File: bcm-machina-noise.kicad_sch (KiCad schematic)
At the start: 61 parts, among them J1 USB_A, J2 AVR-ISP-6, J3 AudioJack2_Ground, J4 AudioJack2_Ground, Q1 2N5457, Q2 2N5457, SW1 SW_Push, SW2 SW_Push, U1 4069, U2 MCP602, U3 ATtiny84V-10P

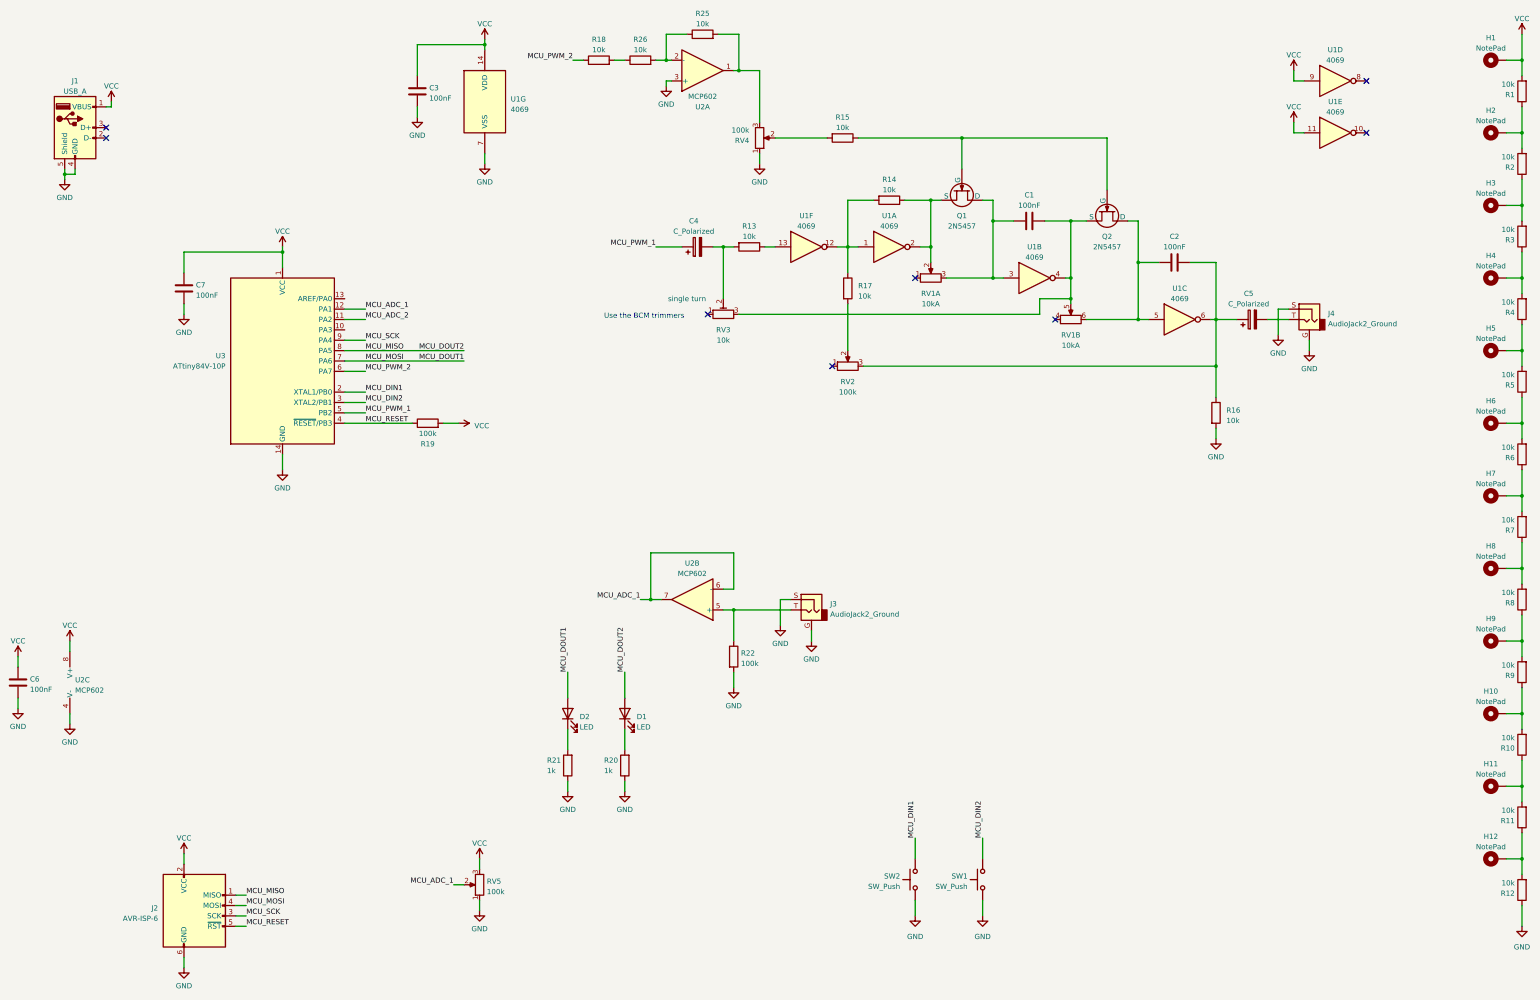
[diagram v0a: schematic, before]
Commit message: fixed errors
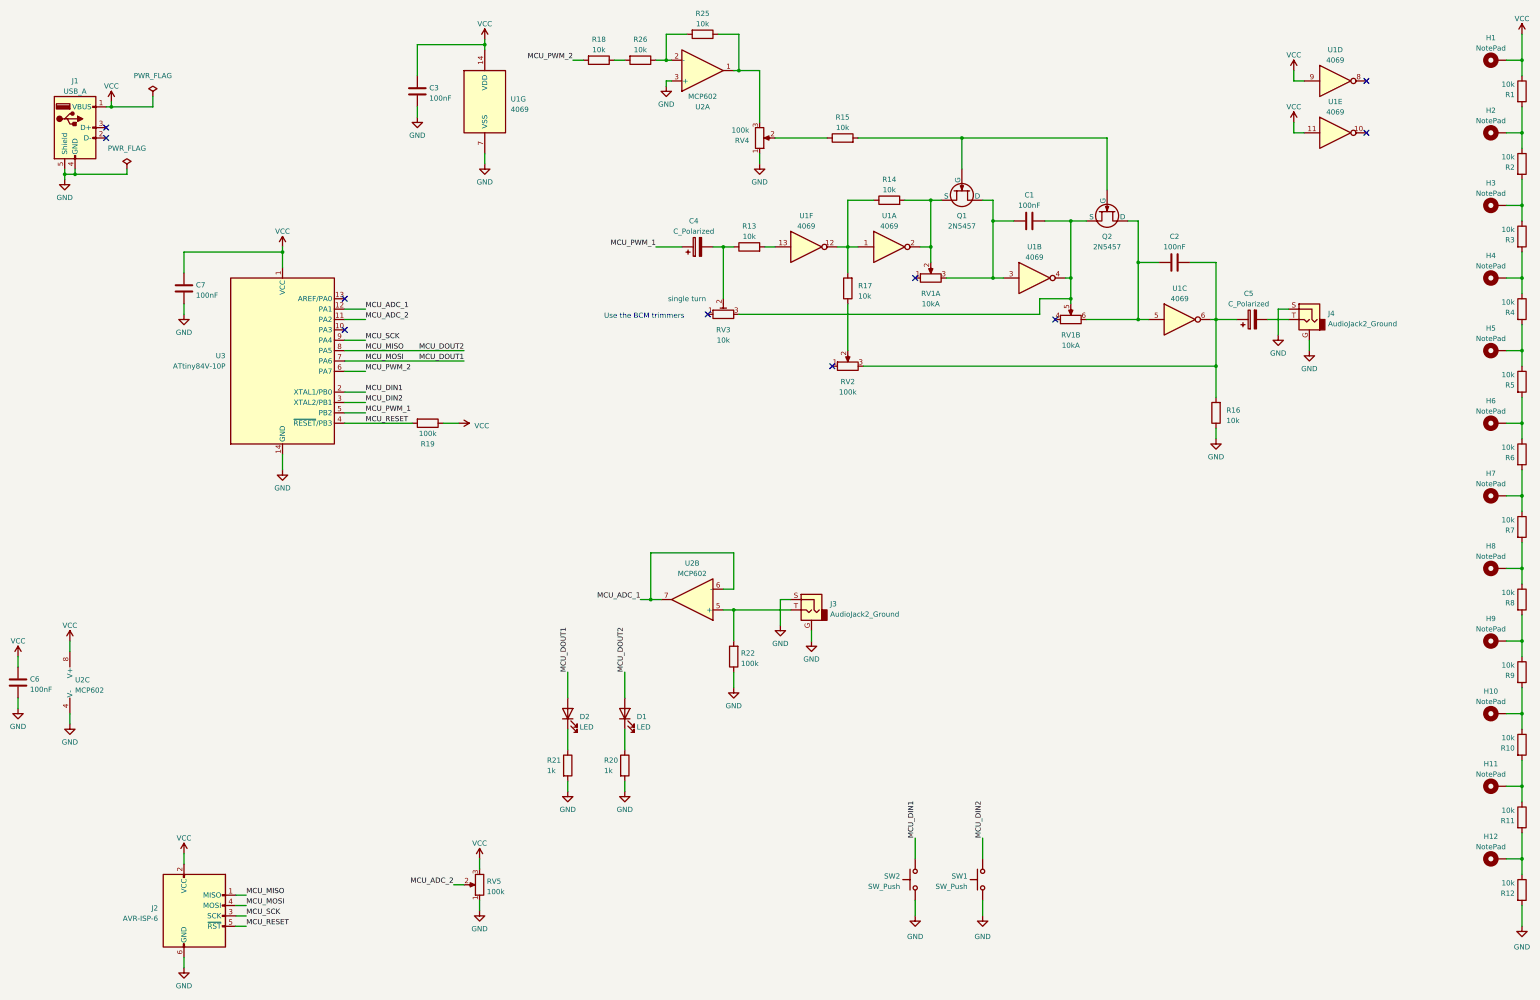
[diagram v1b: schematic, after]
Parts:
- C1, C2: symbol Rumblesan Standard Parts:C -> Device:C
- C3, C6, C7: symbol rumblesan-standard-parts:C -> Device:C
- C4, C5: symbol Rumblesan Standard Parts:C_Polarized -> Device:C_Polarized
- J3, J4: symbol Connector:AudioJack2_Ground -> Connector_Audio:AudioJack2_Ground
- R1, R10, R11, R12, R2, R20, R21, R22, R3, R4, R5, R6, R7, R8, R9: symbol rumblesan-standard-parts:R -> Device:R
- R13, R14, R15, R16, R17, R18, R19, R25, R26: symbol Rumblesan Standard Parts:R -> Device:R
- RV2, RV4: symbol Rumblesan Standard Parts:R_Potentiometer -> Device:R_Potentiometer
- RV3: symbol Rumblesan Standard Parts:R_Potentiometer_Trim -> Device:R_Potentiometer_Trim
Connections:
- net GND: now also R12.2, R16.1, R20.2, R21.2, R22.1; no longer R12.1, R16.2, R20.1, R21.1, R22.2
- net MCU_ADC_1: no longer RV5.2
- net MCU_ADC_2: now also RV5.2
- net MCU_PWM_2: now also R18.2; no longer R18.1
- net MCU_RESET: now also R19.2; no longer R19.1
- net VCC: now also R1.1, R19.1; no longer R1.2, R19.2
- net at U1.1, U1.12: now also R14.1, R17.2; no longer R14.2, R17.1
- net at Q1.3 (S), RV1.2, U1.2: now also R14.2; no longer R14.1
- net at C2.2, C5.1, RV2.3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: now also R16.2; no longer R16.1
- net at C4.2, RV3.2: now also R13.1; no longer R13.2
- net at U1.13: now also R13.2; no longer R13.1
- net at D2.1 (K): now also R21.1; no longer R21.2
- net at RV4.3, U2.1: now also R25.1; no longer R25.2
- net at R26.1: now also R25.2, U2.2 (-); no longer R18.2
- net at Q1.2 (G), Q2.2 (G): now also R15.2; no longer R15.1
- net at RV4.2: now also R15.1; no longer R15.2
- net at J3.T, U2.5 (+): now also R22.2; no longer R22.1
- net at RV2.2: now also R17.1; no longer R17.2
- net at D1.1 (K): now also R20.1; no longer R20.2
- new net: H11.1, R10.2, R11.1
- new net: H12.1, R11.2, R12.1
- new net: H4.1, R3.2, R4.1
- new net: H8.1, R7.2, R8.1
- new net: H9.1, R8.2, R9.1
- new net: H5.1, R4.2, R5.1
- new net: H6.1, R5.2, R6.1
- new net: H2.1, R1.2, R2.1
- new net: H3.1, R2.2, R3.1
- new net: H7.1, R6.2, R7.1
- new net: H10.1, R10.1, R9.2
- new net: R18.1, R26.2
- no-connect marks 8 -> 10
